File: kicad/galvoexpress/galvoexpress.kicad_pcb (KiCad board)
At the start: 2 copper layers, 29 parts, among them J1 MP1584EN OUT +5V, J10 laser 2, J2 MP1584EN OUT -, J3 MP1584EN IN +15V, J4 MP1584EN IN -, J5 +15V -15V, J6 laser, J7 Screw_Terminal_01x02 5V, J8 Screw_Terminal_01x08, J9 laser 1, Q1 Q_NPN_BEC, U1 WEMOS_D1_mini, U2 MCP4922, U3 LM358, U4 LM358

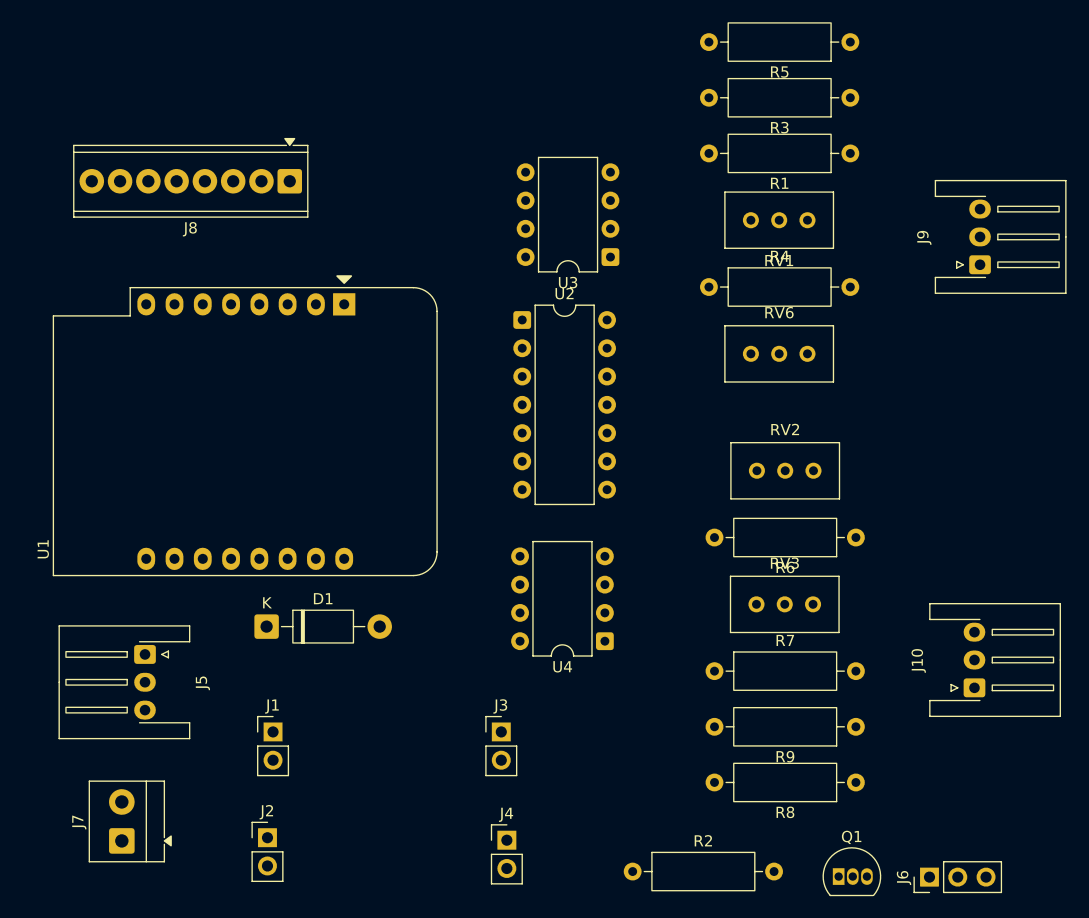
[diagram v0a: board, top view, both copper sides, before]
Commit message: kicad v1.0
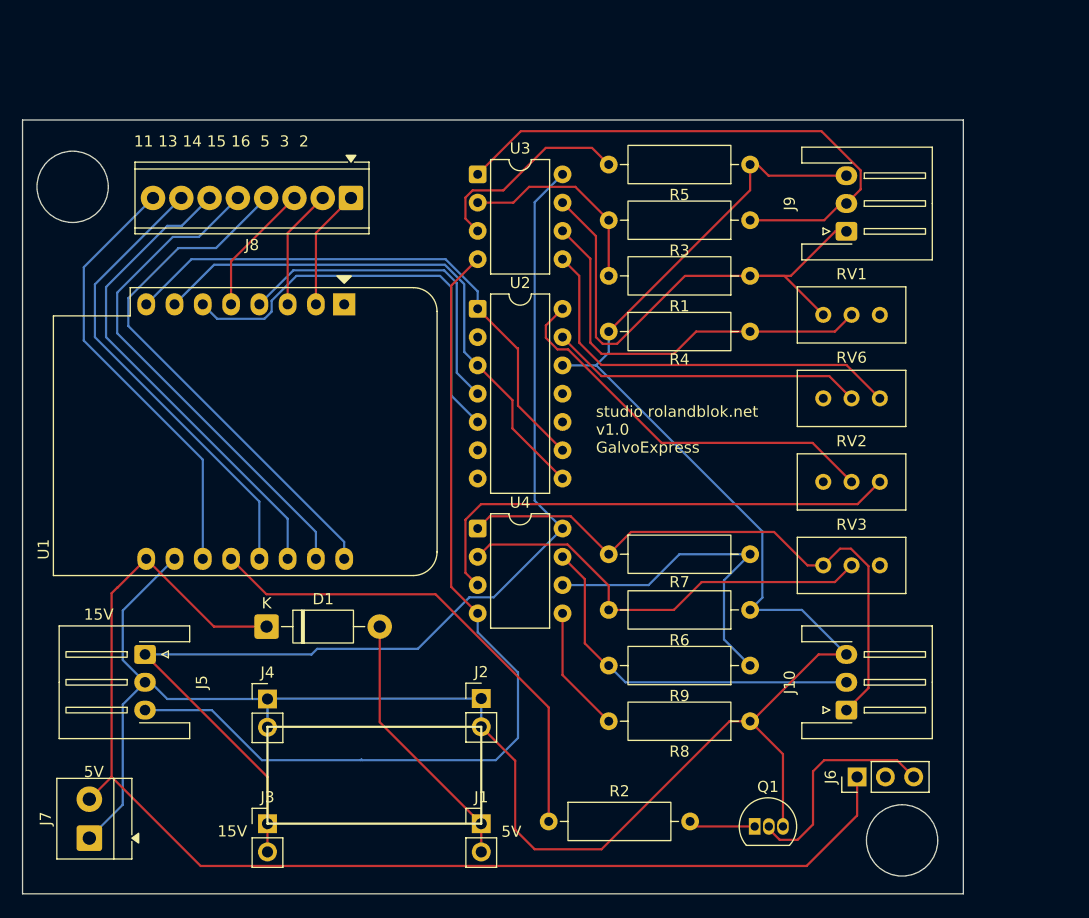
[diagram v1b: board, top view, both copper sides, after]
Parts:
- moved J4 25.0 mm to (75.5, 97.5)
- moved J2 22.9 mm to (94.7, 97.5)
- moved J3 22.6 mm to (75.5, 108.7)
- moved J1 20.4 mm to (94.7, 108.7)
- moved U4 15.3 mm to (94.4, 82.2), turned to 0 degrees
- moved RV1 14.4 mm to (130.5, 63.0), turned to 0 degrees
- moved R1 14.2 mm to (118.8, 59.5)
- moved R3 14.2 mm to (118.8, 54.5)
- moved R5 14.2 mm to (118.8, 49.5)
- moved R7 14.2 mm to (106.2, 84.5)
- moved U3 14.1 mm to (94.4, 50.4), turned to 0 degrees
- moved J9 12.4 mm to (127.5, 55.5)
- moved J10 11.7 mm to (127.5, 98.5)
- moved R6 11.5 mm to (118.8, 89.5)
- moved J6 11.1 mm to (128.5, 104.5)
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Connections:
- J2 pad 1: Net-(J10-Pin_1) -> Net-(J10-Pin_3)
- J2 pad 2: Net-(J10-Pin_1) -> Net-(J10-Pin_3)
- J4 pad 1: Net-(J10-Pin_1) -> Net-(J10-Pin_3)
- J4 pad 2: Net-(J10-Pin_1) -> Net-(J10-Pin_3)
- J5 pad 2: Net-(J10-Pin_1) -> Net-(J10-Pin_3)
- J7 pad 1: Net-(J10-Pin_1) -> Net-(J10-Pin_3)
- J9 pad 1: Net-(J10-Pin_1) -> Net-(J9-Pin_1)
- J9 pad 3: Net-(J9-Pin_3) -> Net-(J10-Pin_3)
- Q1 pad 3: Net-(J10-Pin_1) -> Net-(J10-Pin_3)
- R1 pad 1: Net-(J9-Pin_3) -> Net-(J9-Pin_1)
- R4 pad 1: Net-(J10-Pin_1) -> Net-(J10-Pin_3)
- R5 pad 1: Net-(J10-Pin_1) -> Net-(J10-Pin_3)
- R6 pad 1: Net-(J10-Pin_1) -> Net-(J10-Pin_3)
- R7 pad 1: Net-(J10-Pin_3) -> Net-(J10-Pin_1)
- R8 pad 1: Net-(J10-Pin_1) -> Net-(J10-Pin_3)
- RV1 pad 3: Net-(J9-Pin_3) -> Net-(J9-Pin_1)
- RV3 pad 3: Net-(J10-Pin_3) -> Net-(J10-Pin_1)
- U1 pad 10: Net-(J10-Pin_1) -> Net-(J10-Pin_3)
- U1 pad 11: Net-(J8-Pin_7) -> Net-(J8-Pin_8)
- U1 pad 13: Net-(J8-Pin_6) -> Net-(J8-Pin_7)
- U1 pad 14: Net-(J8-Pin_5) -> Net-(J8-Pin_6)
- U1 pad 15: Net-(J8-Pin_2) -> Net-(J8-Pin_5)
- U1 pad 16: Net-(J8-Pin_1) -> Net-(J8-Pin_4)
- U1 pad 2: Net-(J8-Pin_3) -> Net-(J8-Pin_1)
- U1 pad 3: Net-(J8-Pin_4) -> Net-(J8-Pin_2)
- U1 pad 5: Net-(J8-Pin_8) -> Net-(J8-Pin_3)
- U2 pad 12: Net-(J10-Pin_1) -> Net-(J10-Pin_3)
- U3 pad 7: Net-(J9-Pin_3) -> Net-(J9-Pin_1)
- U4 pad 1: Net-(J10-Pin_3) -> Net-(J10-Pin_1)
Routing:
- net Net-(J10-Pin_3): track 0.00 -> 199.5 mm
- net Net-(D1-K): track 0.00 -> 112.7 mm
- net Net-(J3-Pin_1): track 0.00 -> 98.4 mm
- net Net-(J5-Pin_3): track 0.00 -> 82.7 mm
- net Net-(J10-Pin_1): track 0.00 -> 54.1 mm
- net Net-(J9-Pin_2): track 0.00 -> 50.2 mm
- net Net-(U1-3V3): track 0.00 -> 50.1 mm
- net Net-(U1-CS/D8): track 0.00 -> 49.3 mm
- net Net-(J9-Pin_1): track 0.00 -> 48.3 mm
- net Net-(J8-Pin_4): track 0.00 -> 47.6 mm
- net Net-(J8-Pin_5): track 0.00 -> 45.7 mm
- net Net-(U4A-+): track 0.00 -> 45.0 mm
- net Net-(U1-D3): track 0.00 -> 44.3 mm
- net Net-(J8-Pin_6): track 0.00 -> 43.8 mm
- net Net-(J8-Pin_7): track 0.00 -> 41.7 mm
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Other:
- board outline added: 84.5 x 69.5 mm
- board text added: "11 13 14 15 16 5 3 2"
- board text added: "15V"
- board text added: "5V"
- board text added: "studio rolandblok.net v1.0 GalvoExpress"
